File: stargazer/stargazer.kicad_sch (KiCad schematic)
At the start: 0 parts

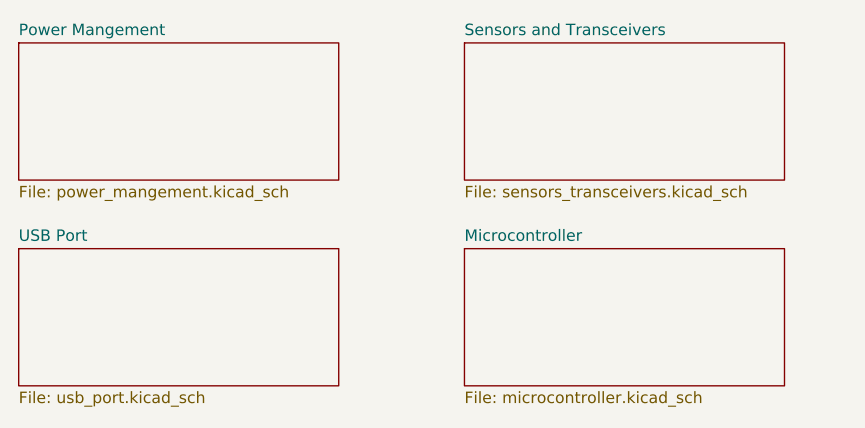
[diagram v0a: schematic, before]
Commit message: New Layout
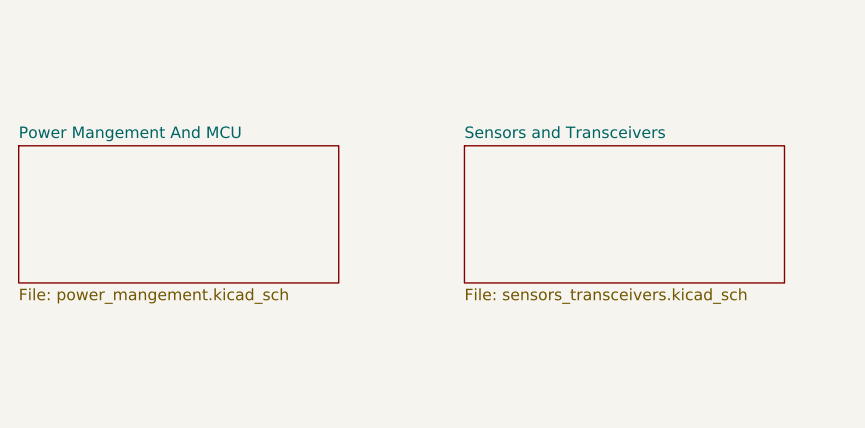
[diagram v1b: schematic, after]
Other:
- sheet Power Mangement renamed Power Mangement And MCU
- removed sheet Microcontroller
- removed sheet USB Port
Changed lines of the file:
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@@
 	)
 	(sheet
-		(at 157.48 77.47)
+		(at 157.48 88.9)
 		(size 35.56 15.24)
 		(fields_autoplaced yes)
@@
 		)
 		(property "Sheetname" "Sensors and Transceivers"
-			(at 157.48 76.7584 0)
+			(at 157.48 88.1884 0)
 			(effects
 				(font
@@
 		)
 		(property "Sheetfile" "sensors_transceivers.kicad_sch"
-			(at 157.48 93.2946 0)
+			(at 157.48 104.7246 0)
 			(effects
 				(font
@@
 	)
 	(sheet
-		(at 107.95 100.33)
+		(at 107.95 88.9)
 		(size 35.56 15.24)
 		(fields_autoplaced yes)
@@
 			(color 0 0 0 0.0000)
 		)
-		(property "Sheetname" "USB Port"
-			(at 107.95 99.6184 0)
-			(effects
-				(font
-					(size 1.27 1.27)
-				)
-				(justify left bottom)
-			)
-		)
-		(property "Sheetfile" "usb_port.kicad_sch"
-			(at 107.95 116.1546 0)
-			(effects
-				(font
-					(size 1.27 1.27)
-				)
-				(justify left top)
-			)
-		)
-		(instances
-			(project "stargazer"
-				(path "/a232d2e9-9a56-4311-b00b-a3ecc9fa3c35"
-					(page "5")
-				)
-			)
-		)
-	)
-	(sheet
-		(at 107.95 77.47)
-		(size 35.56 15.24)
-		(fields_autoplaced yes)
-		(stroke
-			(width 0.1524)
-			(type solid)
-		)
-		(fill
-			(color 0 0 0 0.0000)
-		)
-		(property "Sheetname" "Power Mangement"
-			(at 107.95 76.7584 0)
+		(property "Sheetname" "Power Mangement And MCU"
+			(at 107.95 88.1884 0)
 			(effects
 				(font
@@
 		)
 		(property "Sheetfile" "power_mangement.kicad_sch"
-			(at 107.95 93.2946 0)
+			(at 107.95 104.7246 0)
 			(effects
 				(font
@@
 				)
 			)
-		)
-	)
-	(sheet
-		(at 157.48 100.33)
-		(size 35.56 15.24)
-		(fields_autoplaced yes)
-		(stroke
-			(width 0.1524)
-			(type solid)
-		)
-		(fill
-			(color 0 0 0 0.0000)
-		)
-		(property "Sheetname" "Microcontroller"
-			(at 157.48 99.6184 0)
-			(effects
-				(font
-					(size 1.27 1.27)
-				)
-				(justify left bottom)
-			)
-		)
-		(property "Sheetfile" "microcontroller.kicad_sch"
-			(at 157.48 116.1546 0)
-			(effects
-				(font
-					(size 1.27 1.27)
-				)
-				(justify left top)
-			)
-		)
-		(instances
-			(project "stargazer"
-				(path "/a232d2e9-9a56-4311-b00b-a3ecc9fa3c35"
-					(page "3")
-				)
-			)
